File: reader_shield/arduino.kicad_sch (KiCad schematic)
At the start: 1 part

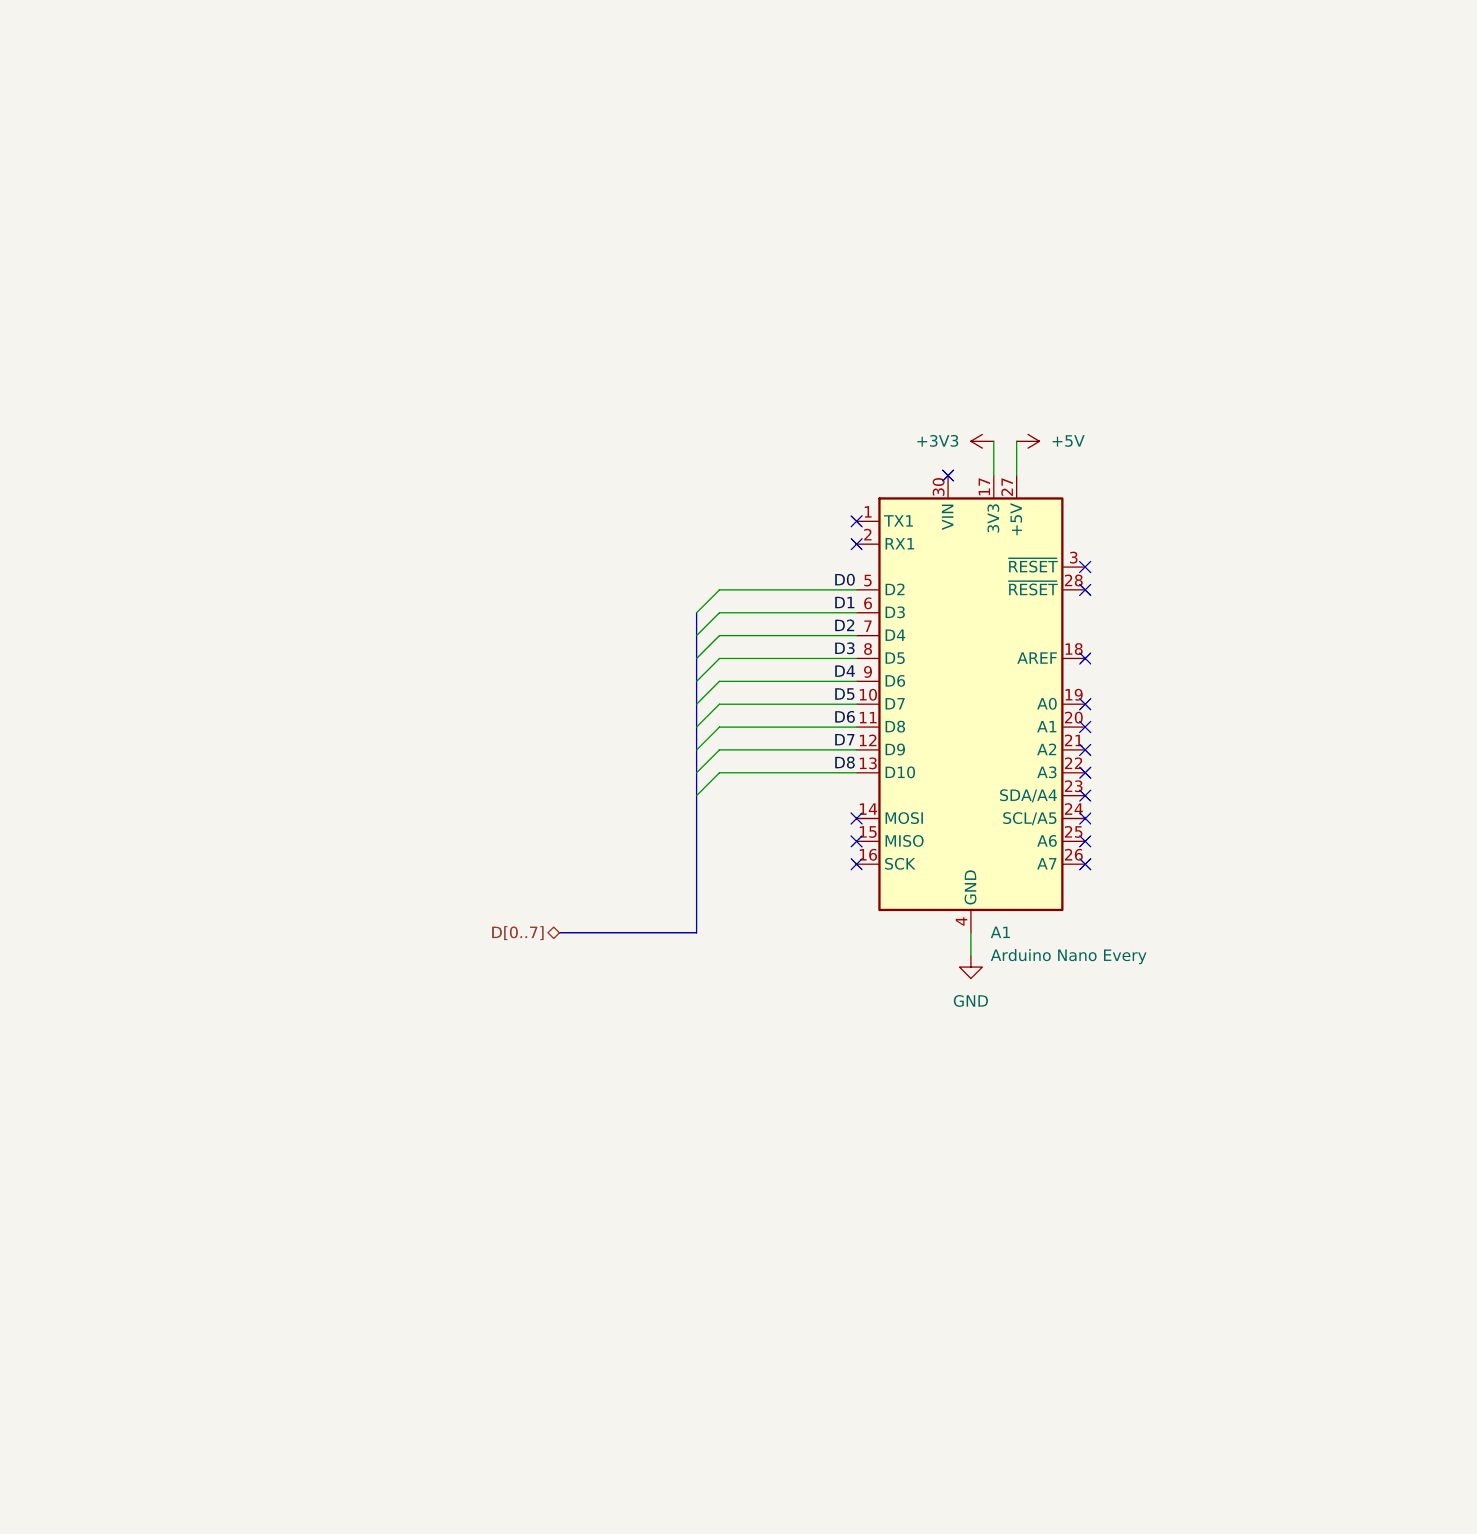
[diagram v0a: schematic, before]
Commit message: Revisions 1 and 2
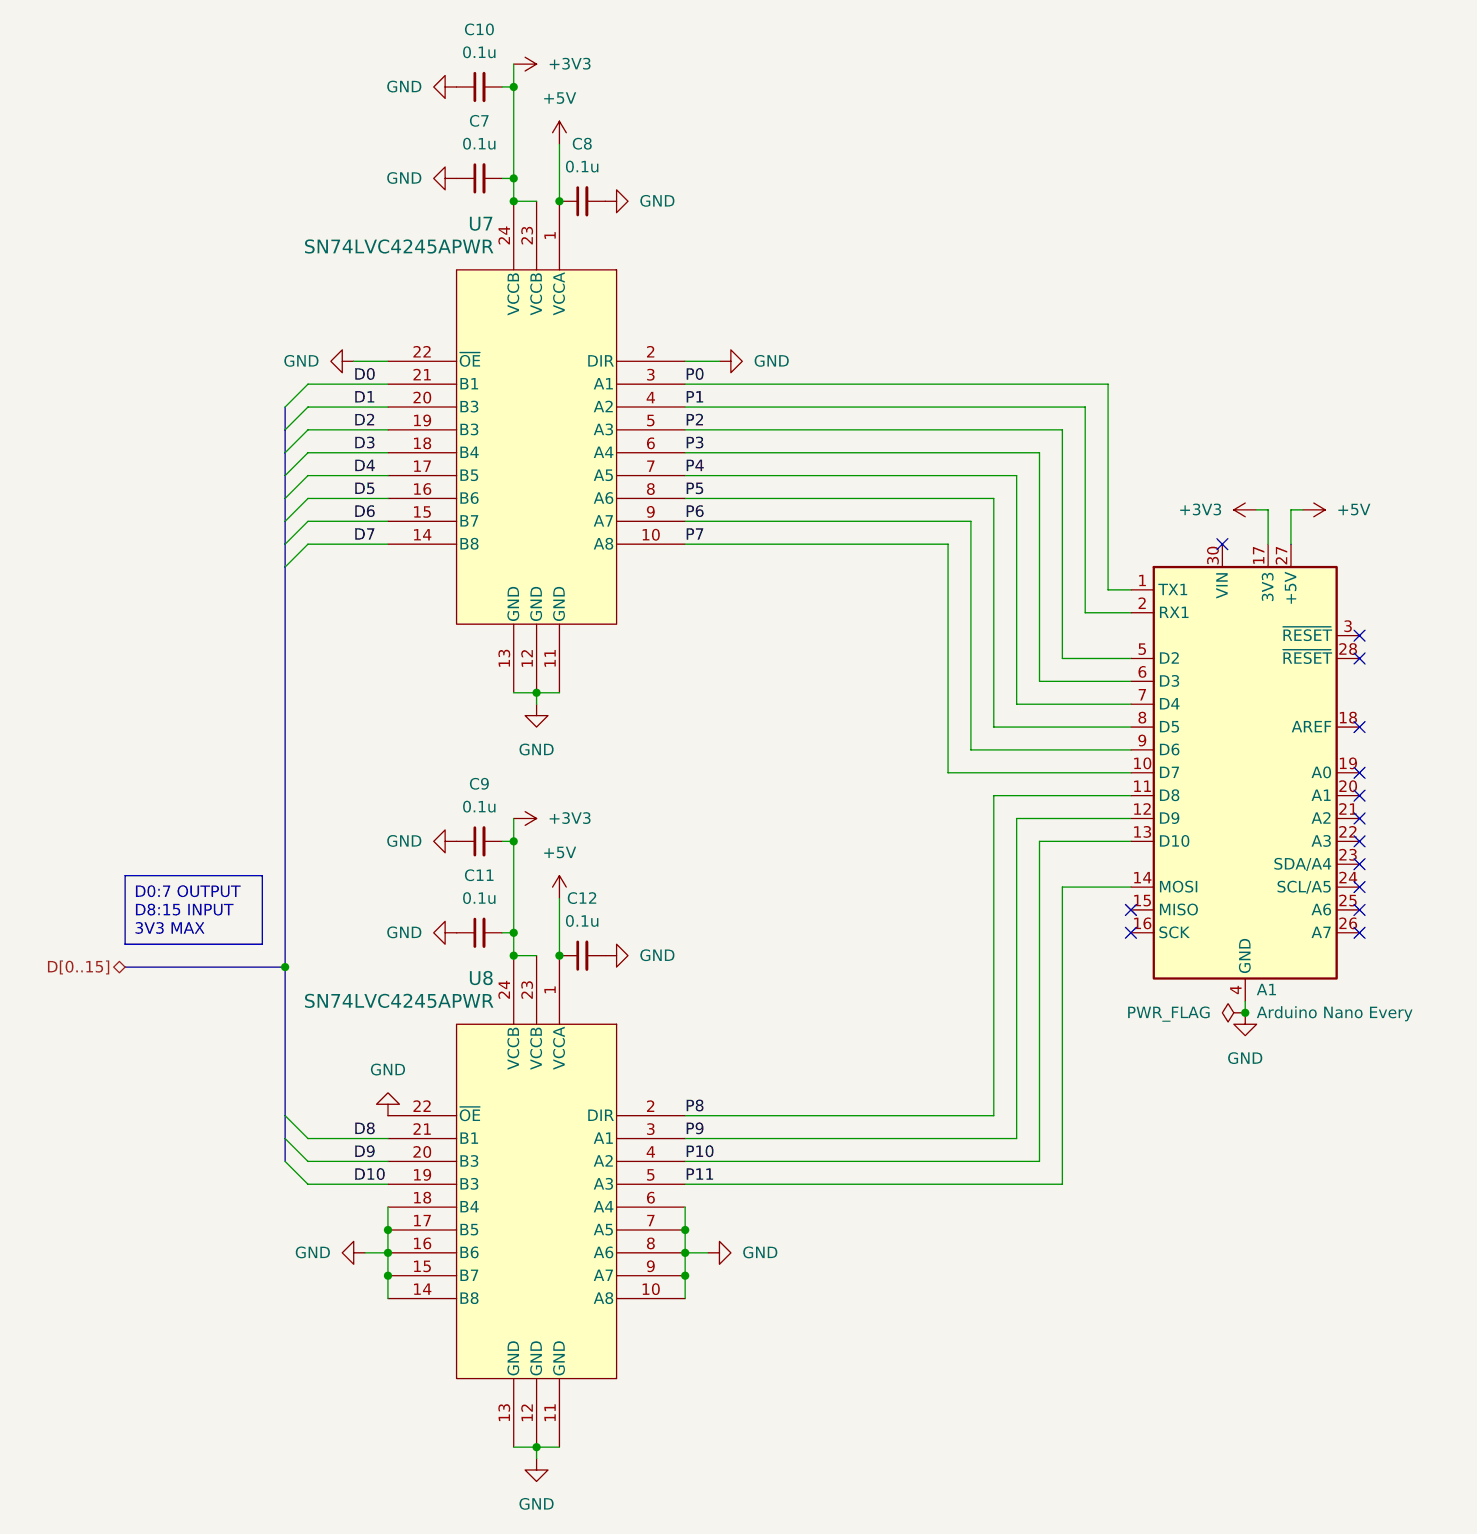
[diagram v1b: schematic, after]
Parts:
- added C10, C11, C12, C7, C8, C9: 0.1u, Capacitor_SMD:C_0402_1005Metric, symbol Device:C_Small
- added U7, U8: SN74LVC4245APWR, Package_SO:TSSOP-24_4.4x6.5mm_P0.5mm, symbol reader_flash:SN74LVC4245APWR
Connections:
- net +3V3: now also C10.2, C11.2, C7.2, C9.2, U7.23 (VCCB), U7.24 (VCCB), U8.23 (VCCB), U8.24 (VCCB)
- net +5V: now also C12.1, C8.1, U7.1 (VCCA), U8.1 (VCCA)
- net D0: now also U7.21 (B1); no longer A1.5 (D2)
- net D1: now also U7.20 (B3); no longer A1.6 (D3)
- net D2: now also U7.19 (B3); no longer A1.7 (D4)
- net D3: now also U7.18 (B4); no longer A1.8 (D5)
- net D4: now also U7.17 (B5); no longer A1.9 (D6)
- net D5: now also U7.16 (B6); no longer A1.10 (D7)
- net D6: now also U7.15 (B7); no longer A1.11 (D8)
- net D7: now also U7.14 (B8); no longer A1.12 (D9)
- net D8: now also U8.21 (B1); no longer A1.13 (D10)
- net GND: now also C10.1, C11.1, C12.2, C7.1, C8.2, C9.1, U7.11 (GND), U7.12 (GND), U7.13 (GND), U7.2 (DIR), U7.22 (~{OE}), U8.10 (A8), U8.11 (GND), U8.12 (GND), U8.13 (GND), U8.14 (B8), U8.15 (B7), U8.16 (B6), U8.17 (B5), U8.18 (B4), U8.22 (~{OE}), U8.6 (A4), U8.7 (A5), U8.8 (A6), U8.9 (A7)
- net P0: now reaches A1.1 (TX1)
- net P0: now also U7.3 (A1)
- net P11: now reaches A1.14 (MOSI)
- net P11: now also U8.5 (A3)
- net P1: now reaches A1.2 (RX1)
- net P1: now also U7.4 (A2)
- new net D10: U8.19 (B3)
- new net D9: U8.20 (B3)
- new net P10: A1.13 (D10), U8.4 (A2)
- new net P2: A1.5 (D2), U7.5 (A3)
- new net P3: A1.6 (D3), U7.6 (A4)
- new net P4: A1.7 (D4), U7.7 (A5)
- new net P5: A1.8 (D5), U7.8 (A6)
- new net P6: A1.9 (D6), U7.9 (A7)
- new net P7: A1.10 (D7), U7.10 (A8)
- new net P8: A1.11 (D8), U8.2 (DIR)
- new net P9: A1.12 (D9), U8.3 (A1)
- no-connect marks 17 -> 14
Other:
- moved on the sheet: A1
